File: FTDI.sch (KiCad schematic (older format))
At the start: 4 parts, among them U2 FT232RL

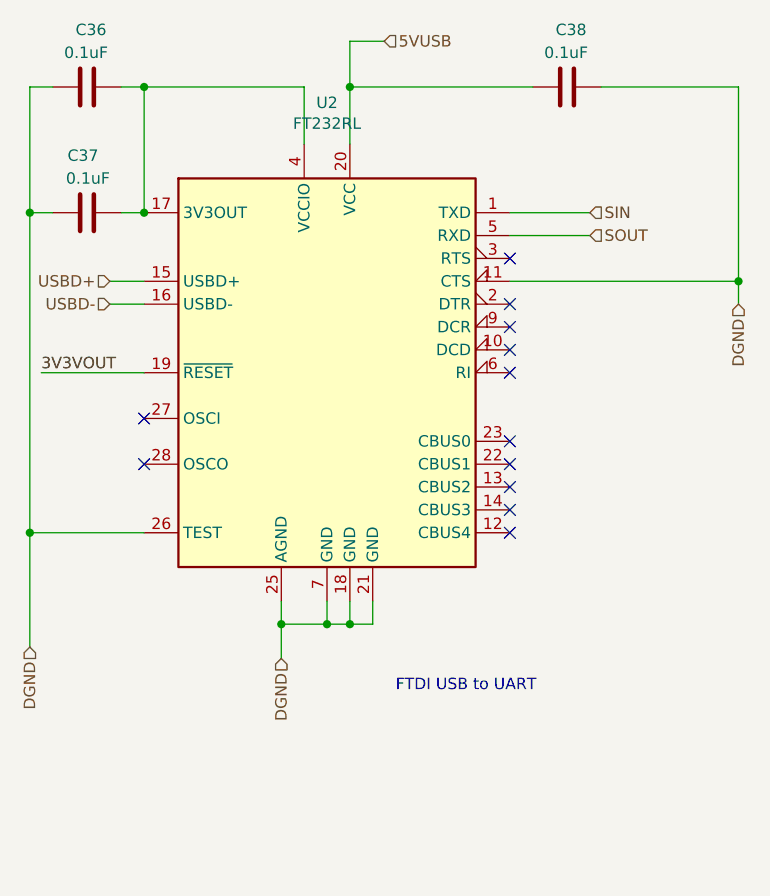
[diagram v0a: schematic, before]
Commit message: first draft done, needs reviewing
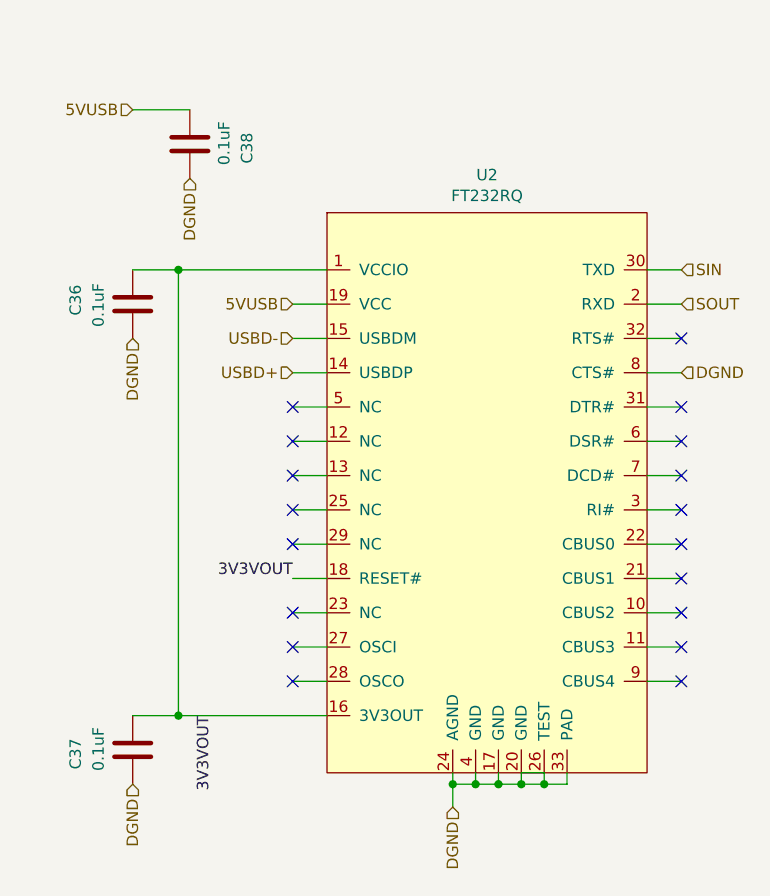
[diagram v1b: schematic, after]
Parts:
- removed U2: FT232RL, Package_SO:SSOP-28_5.3x10.2mm_P0.65mm, symbol Interface_USB:FT232RL
- added U2: FT232RQ, Package_DFN_QFN:QFN-32-1EP_5x5mm_P0.5mm_EP3.3x3.3mm, symbol SIB_Footprint:FT232RQ
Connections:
- net 3V3VOUT: now also C36.1, C37.2, U2.1 (VCCIO), U2.16 (3V3OUT), U2.18 (RESET#)
- net 5VUSB: now also U2.19 (VCC)
- net DGND: now also U2.17 (GND), U2.20 (GND), U2.24 (AGND), U2.26 (TEST), U2.33 (PAD), U2.4 (GND), U2.8 (CTS#)
- net SIN: now also U2.30 (TXD)
- net SOUT: now also U2.2 (RXD)
- net USBD+: now also U2.14 (USBDP)
- net USBD-: now also U2.15 (USBDM)
- no-connect marks 12 -> 18
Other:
- note removed: "FTDI USB to UART"
- moved on the sheet: C36, C37, C38
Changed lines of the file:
@@
 L Device:C C?
 U 1 1 5E190CFD
-P 6150 1950
+P 4500 2200
 AR Path="/5E190CFD" Ref="C?"  Part="1"
 AR Path="/5E18BB0B/5E190CFD" Ref="C?"  Part="1"
 AR Path="/5EBF9349/5E190CFD" Ref="C38"  Part="1"
-F 0 "C38" V 5900 1900 50  0000 L CNN
-F 1 "0.1uF" V 6000 1850 50  0000 L CNN
-F 2 "Capacitor_SMD:C_0402_1005Metric" H 6188 1800 50  0001 C CNN
-F 3 "~" H 6150 1950 50  0001 C CNN
-	1    6150 1950
-	0    1    1    0
+F 0 "C38" V 4250 2150 50  0000 L CNN
+F 1 "0.1uF" V 4350 2100 50  0000 L CNN
+F 2 "Capacitor_SMD:C_0402_1005Metric" H 4538 2050 50  0001 C CNN
+F 3 "~" H 4500 2200 50  0001 C CNN
+	1    4500 2200
+	-1   0    0    1
 $EndComp
-$Comp
-L Interface_USB:FT232RL U?
-U 1 1 5E190D03
-P 5100 3200
-AR Path="/5E190D03" Ref="U?"  Part="1"
-AR Path="/5E18BB0B/5E190D03" Ref="U?"  Part="1"
-AR Path="/5EBF9349/5E190D03" Ref="U2"  Part="1"
-F 0 "U2" H 5100 4381 50  0000 C CNN
-F 1 "FT232RL" H 5100 4290 50  0000 C CNN
-F 2 "Package_SO:SSOP-28_5.3x10.2mm_P0.65mm" H 6200 2300 50  0001 C CNN
-F 3 "https://www.ftdichip.com/Support/Documents/DataSheets/ICs/DS_FT232R.pdf" H 5100 3200 50  0001 C CNN
-	1    5100 3200
-	1    0    0    -1
-$EndComp
-Wire Wire Line
-	4900 4200 4900 4300
-Wire Wire Line
-	4900 4300 5100 4300
-Wire Wire Line
-	5100 4300 5100 4200
-Connection ~ 4900 4300
-Wire Wire Line
-	4900 4300 4900 4450
-Wire Wire Line
-	5100 4300 5200 4300
-Wire Wire Line
-	5200 4300 5200 4200
-Connection ~ 5100 4300
-Wire Wire Line
-	5200 4300 5300 4300
-Wire Wire Line
-	5300 4300 5300 4200
-Connection ~ 5200 4300
-NoConn ~ 4300 3400
-NoConn ~ 4300 3600
-Wire Wire Line
-	4300 3900 3800 3900
-Connection ~ 3800 3900
-Wire Wire Line
-	3800 3900 3800 4400
-Wire Wire Line
-	4300 3200 3850 3200
 $Comp
 L Device:C C?
 U 1 1 5E190D1F
-P 4050 1950
+P 4250 2900
 AR Path="/5E190D1F" Ref="C?"  Part="1"
 AR Path="/5E18BB0B/5E190D1F" Ref="C?"  Part="1"
 AR Path="/5EBF9349/5E190D1F" Ref="C36"  Part="1"
-F 0 "C36" V 3800 1900 50  0000 L CNN
-F 1 "0.1uF" V 3900 1850 50  0000 L CNN
-F 2 "Capacitor_SMD:C_0402_1005Metric" H 4088 1800 50  0001 C CNN
-F 3 "~" H 4050 1950 50  0001 C CNN
-	1    4050 1950
-	0    1    1    0
+F 0 "C36" V 4000 2850 50  0000 L CNN
+F 1 "0.1uF" V 4100 2800 50  0000 L CNN
+F 2 "Capacitor_SMD:C_0402_1005Metric" H 4288 2750 50  0001 C CNN
+F 3 "~" H 4250 2900 50  0001 C CNN
+	1    4250 2900
+	1    0    0    -1
 $EndComp
-NoConn ~ 5900 3500
-NoConn ~ 5900 3600
-NoConn ~ 5900 3700
-NoConn ~ 5900 3800
-NoConn ~ 5900 3900
-NoConn ~ 5900 2700
-NoConn ~ 5900 2900
-NoConn ~ 5900 3000
-NoConn ~ 5900 3100
-NoConn ~ 5900 3200
-Wire Wire Line
-	6250 2500 5900 2500
-Wire Wire Line
-	5900 2600 6250 2600
-Wire Wire Line
-	5350 1750 5200 1750
-Wire Wire Line
-	5200 1750 5200 1950
-Connection ~ 5200 1950
-Wire Wire Line
-	5200 1950 5200 2200
-Wire Wire Line
-	5000 1950 5000 2200
-Wire Wire Line
-	6900 1950 6900 2800
-Connection ~ 6900 2800
-Wire Wire Line
-	6900 2800 6900 2900
-Wire Wire Line
-	5900 2800 6900 2800
-Text Notes 5400 4600 0    50   ~ 0
-FTDI USB to UART
 $Comp
 L Device:C C?
 U 1 1 5E190D4F
-P 4050 2500
+P 4250 4850
 AR Path="/5E190D4F" Ref="C?"  Part="1"
 AR Path="/5E18BB0B/5E190D4F" Ref="C?"  Part="1"
 AR Path="/5EBF9349/5E190D4F" Ref="C37"  Part="1"
-F 0 "C37" V 4300 2450 50  0000 L CNN
-F 1 "0.1uF" V 4200 2400 50  0000 L CNN
-F 2 "Capacitor_SMD:C_0402_1005Metric" H 4088 2350 50  0001 C CNN
-F 3 "~" H 4050 2500 50  0001 C CNN
-	1    4050 2500
-	0    -1   -1   0
+F 0 "C37" V 4500 4800 50  0000 L CNN
+F 1 "0.1uF" V 4400 4750 50  0000 L CNN
+F 2 "Capacitor_SMD:C_0402_1005Metric" H 4288 4700 50  0001 C CNN
+F 3 "~" H 4250 4850 50  0001 C CNN
+	1    4250 4850
+	-1   0    0    1
 $EndComp
+$Comp
+L SIB_Footprint:FT232RQ U2
+U 1 1 601E1423
+P 5800 3650
+F 0 "U2" H 5800 4965 50  0000 C CNN
+F 1 "FT232RQ" H 5800 4874 50  0000 C CNN
+F 2 "Package_DFN_QFN:QFN-32-1EP_5x5mm_P0.5mm_EP3.3x3.3mm" H 5800 3650 50  0001 C CNN
+F 3 "" H 5800 3650 50  0001 C CNN
+	1    5800 3650
+	1    0    0    -1
+$EndComp
+Text HLabel 6650 2750 2    50   Input ~ 0
+SIN
+Text HLabel 6650 2900 2    50   Input ~ 0
+SOUT
 Wire Wire Line
-	4150 2900 4300 2900
+	6500 2750 6650 2750
 Wire Wire Line
-	4150 2800 4300 2800
+	6500 2900 6650 2900
+Text HLabel 6650 3200 2    50   Input ~ 0
+DGND
 Wire Wire Line
-	4300 1950 5000 1950
+	6650 3200 6500 3200
+NoConn ~ 6650 3050
 Wire Wire Line
-	4300 2500 4300 1950
-Connection ~ 4300 1950
+	6500 3050 6650 3050
+NoConn ~ 6650 3350
+NoConn ~ 6650 3500
+NoConn ~ 6650 3650
+NoConn ~ 6650 3800
+NoConn ~ 6650 3950
+NoConn ~ 6650 4100
+NoConn ~ 6650 4250
+NoConn ~ 6650 4400
+NoConn ~ 6650 4550
 Wire Wire Line
-	4200 1950 4300 1950
+	6650 3350 6500 3350
 Wire Wire Line
-	3900 1950 3800 1950
+	6650 3500 6500 3500
 Wire Wire Line
-	4200 2500 4300 2500
-Connection ~ 4300 2500
+	6650 3650 6500 3650
 Wire Wire Line
-	3800 1950 3800 2500
+	6650 3800 6500 3800
 Wire Wire Line
-	3900 2500 3800 2500
-Connection ~ 3800 2500
+	6650 3950 6500 3950
 Wire Wire Line
-	3800 2500 3800 3900
+	6500 4100 6650 4100
 Wire Wire Line
-	5200 1950 6000 1950
+	6650 4250 6500 4250
 Wire Wire Line
-	6300 1950 6900 1950
-Text HLabel 4150 2800 0    50   Input ~ 0
+	6650 4400 6500 4400
+Wire Wire Line
+	6650 4550 6500 4550
+NoConn ~ 4950 3350
+NoConn ~ 4950 3500
+NoConn ~ 4950 3650
+NoConn ~ 4950 3800
+NoConn ~ 4950 3950
+NoConn ~ 4950 4250
+NoConn ~ 4950 4400
+NoConn ~ 4950 4550
+Wire Wire Line
+	4950 3350 5100 3350
+Wire Wire Line
+	4950 3500 5100 3500
+Wire Wire Line
+	4950 3650 5100 3650
+Wire Wire Line
+	4950 3800 5100 3800
+Wire Wire Line
+	4950 3950 5100 3950
+Wire Wire Line
+	4950 4250 5100 4250
+Wire Wire Line
+	4950 4400 5100 4400
+Wire Wire Line
+	4950 4550 5100 4550
+Text Label 4950 4100 2    50   ~ 0
+3V3VOUT
+Wire Wire Line
+	5100 4100 4950 4100
+Text HLabel 4950 3200 0    50   Input ~ 0
 USBD+
-Text HLabel 4150 2900 0    50   Input ~ 0
+Text HLabel 4950 3050 0    50   Input ~ 0
 USBD-
-Text HLabel 6250 2500 2    50   Input ~ 0
-SIN
-Text HLabel 6250 2600 2    50   Input ~ 0
-SOUT
-Text Label 3850 3200 0    50   ~ 0
+Wire Wire Line
+	4950 3050 5100 3050
+Wire Wire Line
+	4950 3200 5100 3200
+Wire Wire Line
+	5100 2750 4450 2750
+Wire Wire Line
+	4450 2750 4450 4700
+Wire Wire Line
+	4450 4700 5100 4700
+Wire Wire Line
+	4250 4700 4450 4700
+Connection ~ 4450 4700
+Wire Wire Line
+	4450 2750 4250 2750
+Connection ~ 4450 2750
+Text HLabel 4250 5000 3    50   Input ~ 0
+DGND
+Text HLabel 4250 3050 3    50   Input ~ 0
+DGND
+Text HLabel 5650 5100 3    50   Input ~ 0
+DGND
+Wire Wire Line
+	5650 4950 5650 5000
+Wire Wire Line
+	5650 5000 5750 5000
+Wire Wire Line
+	5750 5000 5750 4950
+Connection ~ 5650 5000
+Wire Wire Line
+	5650 5000 5650 5100
+Wire Wire Line
+	5750 5000 5850 5000
+Wire Wire Line
+	5850 5000 5850 4950
+Connection ~ 5750 5000
+Wire Wire Line
+	5850 5000 5950 5000
+Wire Wire Line
+	5950 5000 5950 4950
+Connection ~ 5850 5000
+Wire Wire Line
+	5950 4950 6050 4950
+Wire Wire Line
+	6050 4950 6050 5000
+Wire Wire Line
+	6050 5000 5950 5000
+Connection ~ 5950 5000
+Text HLabel 4950 2900 0    50   Input ~ 0
+5VUSB
+Wire Wire Line
+	4950 2900 5100 2900
+Text HLabel 4250 2050 0    50   Input ~ 0
+5VUSB
+Text HLabel 4500 2350 3    50   Input ~ 0
+DGND
+Wire Wire Line
+	4250 2050 4500 2050
+Text Label 4600 4700 3    50   ~ 0
 3V3VOUT
-Text HLabel 5350 1750 2    50   Input ~ 0
-5VUSB
-Text HLabel 6900 2900 3    50   Input ~ 0
-DGND
-Text HLabel 4900 4450 3    50   Input ~ 0
-DGND
-Text HLabel 3800 4400 3    50   Input ~ 0
-DGND
+Wire Wire Line
+	6150 4950 6150 5000
+Wire Wire Line
+	6150 5000 6050 5000
+Connection ~ 6050 5000
 $EndSCHEMATC
